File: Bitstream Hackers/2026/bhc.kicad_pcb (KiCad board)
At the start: 2 copper layers, 20 x 20 mm, 7 parts, among them U1 AT24CS01-SSHM

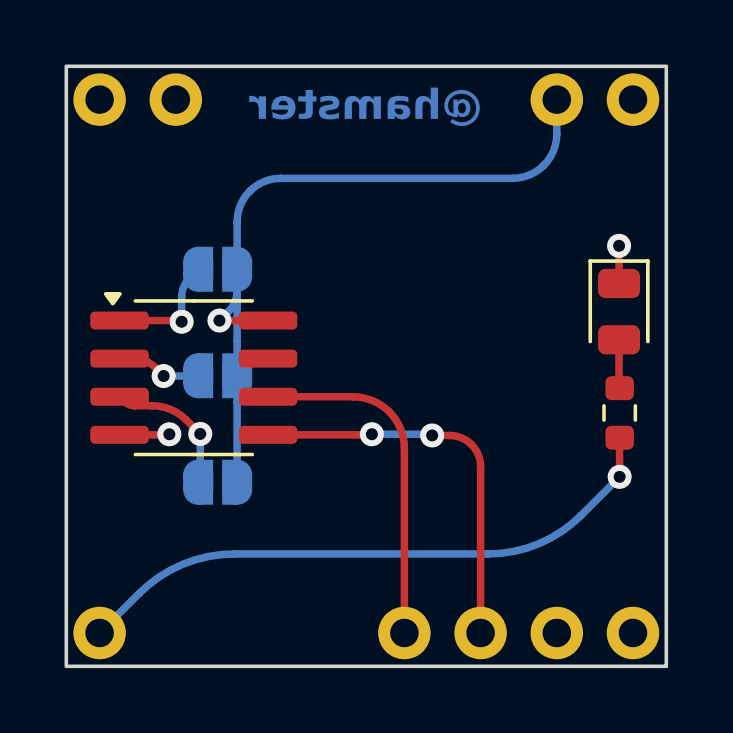
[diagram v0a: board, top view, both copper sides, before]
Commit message: Adding finals, gerbers
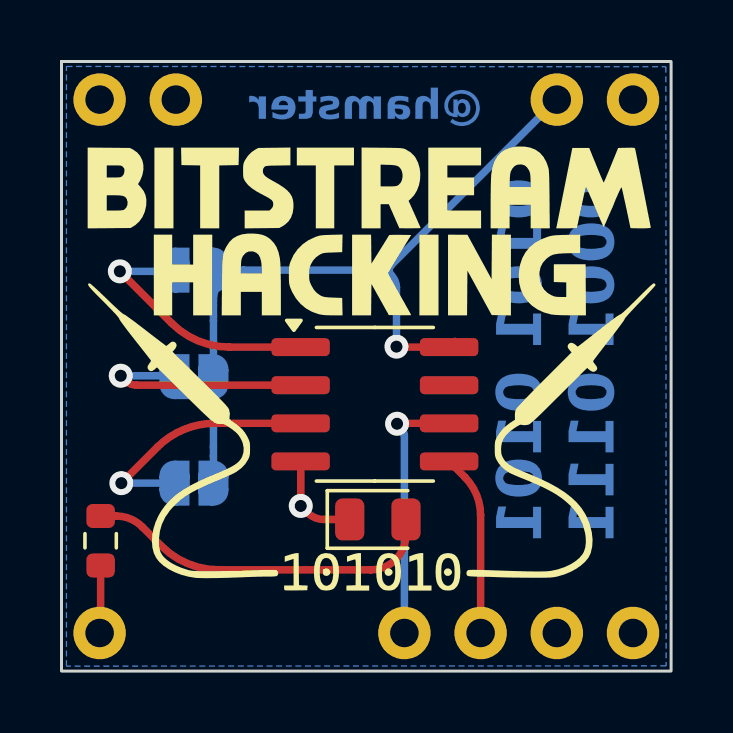
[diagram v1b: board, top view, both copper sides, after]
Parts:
- added G***: LOGO, lib_fp:silkscreen, F.Cu at (106.5, 85.6)
- moved R1 17.8 mm to (97.6, 91.7)
- moved D1 10.6 mm to (106.8, 90.9), turned to 0 degrees
- moved U1 6.10 mm to (106.7, 87.1)
- moved JP1 0.79 mm to (100.7, 82.6)
- moved JP2 0.79 mm to (100.7, 86.2)
- moved JP3 0.79 mm to (100.7, 89.7)
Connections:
- MB1 pad 8: unconnected-(MB1-GND-Pad8) -> GND
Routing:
- net Net-(MB1-CLK): track 20.4 -> 2.26 mm, vias 1 -> 0
- net Net-(D1-A): track 1.62 -> 11.9 mm
- net Net-(MB1-SDA): track 13.2 -> 6.07 mm, vias 2 -> 0
- net Net-(JP2-B): track 2.82 -> 7.93 mm
- net Net-(JP1-B): track 4.05 -> 8.77 mm
- net Net-(JP3-B): track 4.77 -> 8.44 mm
- net Net-(MB1-SCL): track 11.7 -> 9.41 mm, vias 0 -> 1
- net GND: track 3.13 -> 3.47 mm, vias 2 -> 1
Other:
- board size 20 x 20 mm -> 20.3 x 20.3 mm
- board text added: "0101 0101 0001 0111"
